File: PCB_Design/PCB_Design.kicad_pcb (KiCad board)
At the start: 2 copper layers, 54 parts, among them IC1 MIC37303YME, J1 TP4056, J2 632723300011, SW1 SW_Push, SW2 SW_Push, U1 ESP32-WROOM-32

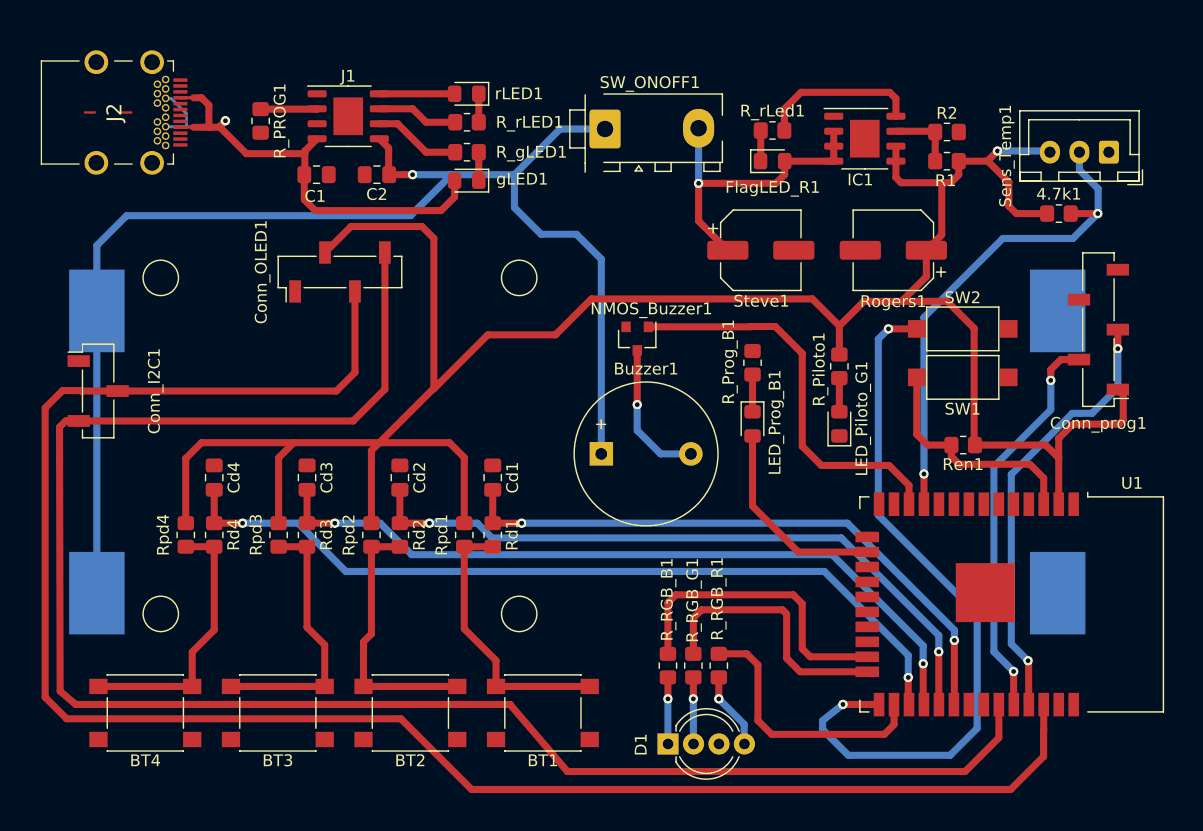
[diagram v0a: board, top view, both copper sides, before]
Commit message: PCB finalizada
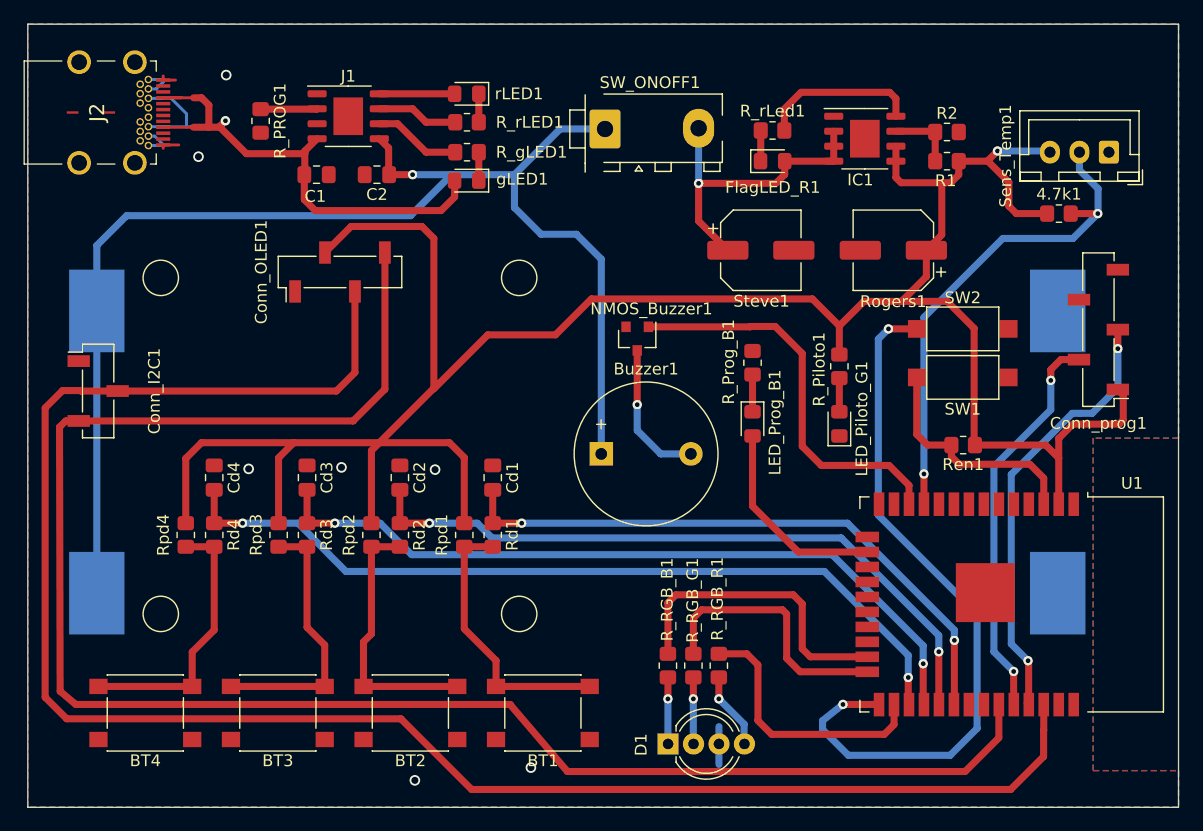
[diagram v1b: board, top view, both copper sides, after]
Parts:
- moved J2 1.46 mm to (66.8, 98.2)
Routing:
- net GND: track 0.00 -> 11.9 mm, vias 0 -> 7
- net Net-(C1-Pad1): track 46.3 -> 53.5 mm
- added copper zone on B.Cu, net GND
- added copper zone on F.Cu, net GND
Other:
- board outline added: 97.6 x 66.4 mm
